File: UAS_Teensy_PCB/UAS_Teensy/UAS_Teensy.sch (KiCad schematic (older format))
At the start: 9 parts, among them J1 UAS-rescue_SM02B-PASS-TBT(LF)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, J2 SM04B-GHS-TB(LF)(SN)-, J3 SM07B-GHS-TB(LF)(SN), J4 SM07B-GHS-TB(LF)(SN), J5 SM04B-GHS-TB(LF)(SN)-, J6 SM04B-GHS-TB(LF)(SN)-, J7 SM04B-GHS-TB(LF)(SN)-, U1 Teensy4.0, U2 BNO055

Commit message: Teensy Board Updates
Teensy Board Updates
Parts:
- J3, J4: footprint JST_SM07B-GHS-TB(LF)(SN) -> UAS_Teensy:JST_SM08B-GHS-TB(LF)(SN)
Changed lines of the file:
@@
 EESchema Schematic File Version 4
+LIBS:UAS_Teensy-cache
 EELAYER 30 0
 EELAYER END
@@
 F 0 "J3" H 3733 2415 50  0000 C CNN
 F 1 "SM07B-GHS-TB(LF)(SN)" H 3733 2324 50  0000 C CNN
-F 2 "JST_SM07B-GHS-TB(LF)(SN)" H 3500 1800 50  0001 L BNN
+F 2 "UAS_Teensy:JST_SM08B-GHS-TB(LF)(SN)" H 3500 1800 50  0001 L BNN
 F 3 "" H 3500 1800 50  0001 L BNN
 F 4 "MANUFACTURER STANDARD" H 3500 1800 50  0001 L BNN "STANDARD"
@@
 F 0 "J4" H 3233 3015 50  0000 C CNN
 F 1 "SM07B-GHS-TB(LF)(SN)" H 3233 2924 50  0000 C CNN
-F 2 "JST_SM07B-GHS-TB(LF)(SN)" H 3000 2400 50  0001 L BNN
+F 2 "UAS_Teensy:JST_SM08B-GHS-TB(LF)(SN)" H 3000 2400 50  0001 L BNN
 F 3 "" H 3000 2400 50  0001 L BNN
 F 4 "MANUFACTURER STANDARD" H 3000 2400 50  0001 L BNN "STANDARD"

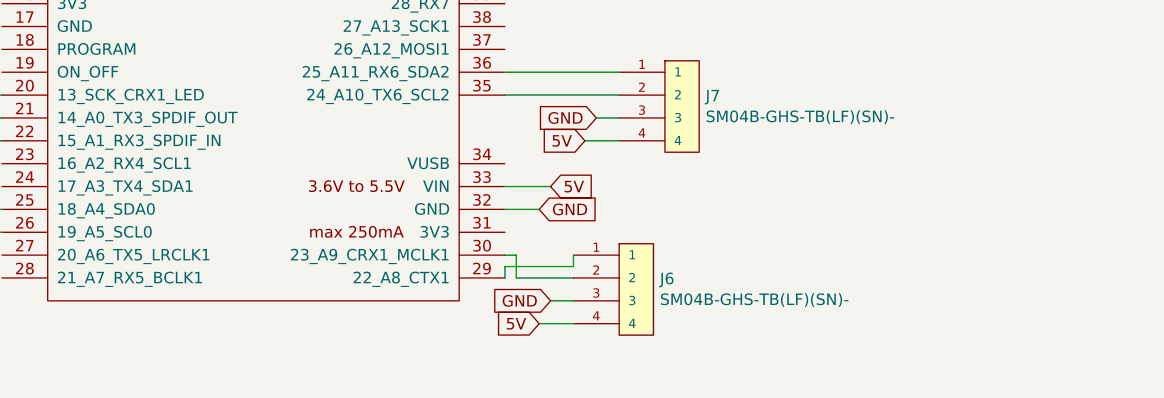
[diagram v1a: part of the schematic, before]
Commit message: For Realsies Final Teensy PCB
lol
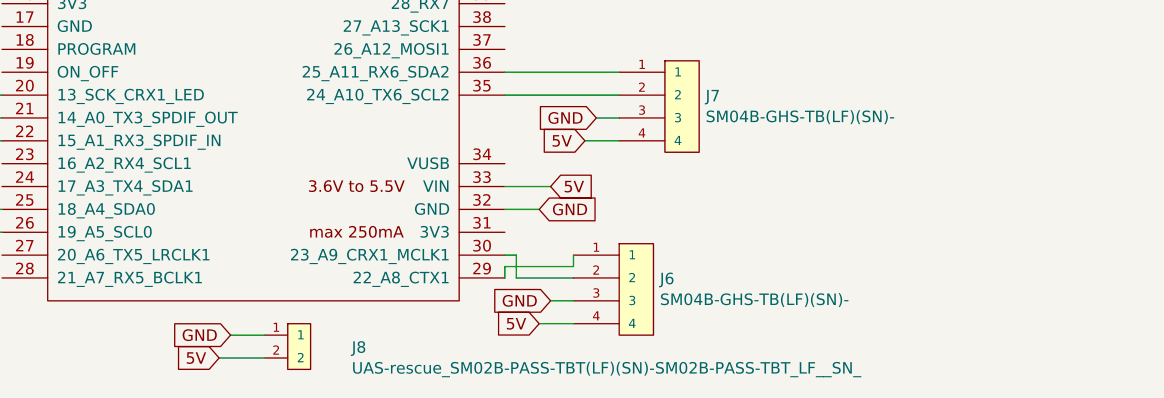
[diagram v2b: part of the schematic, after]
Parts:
- added J8: UAS-rescue_SM02B-PASS-TBT(LF)(SN)-SM02B-PASS-TBT_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, UAS_Teensy:SM02BGHSTBLFSN, symbol UAS:UAS-rescue_SM02B-PASS-TBT(LF)(SN)-SM02B-PASS-TBT_LF__SN_
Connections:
- net +5V: now also J8.2
- net GND: now also J8.1
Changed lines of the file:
@@
 	1    0    0    -1
 $EndComp
-Text GLabel 6550 3700 2    50   Input ~ 0
-5V
-Text GLabel 6500 3800 2    50   Input ~ 0
+Text GLabel 5150 4350 0    50   Input ~ 0
 GND
-Wire Wire Line
-	6550 3700 6350 3700
-Wire Wire Line
-	6500 3800 6350 3800
 Wire Wire Line
 	6750 2700 6750 2800
@@
 	6850 3400 6750 3400
 Wire Wire Line
-	6700 3500 6850 3500
-Wire Wire Line
 	6350 3200 6850 3200
 Wire Wire Line
@@
 Text GLabel 3800 4000 2    50   Input ~ 0
 GND
+$Comp
+L UAS:UAS-rescue_SM02B-PASS-TBT(LF)(SN)-SM02B-PASS-TBT_LF__SN_ J8
+U 1 1 607973F1
+P 5450 4400
+F 0 "J8" H 5680 4396 50  0000 L CNN
+F 1 "UAS-rescue_SM02B-PASS-TBT(LF)(SN)-SM02B-PASS-TBT_LF__SN_" H 5680 4305 50  0000 L CNN
+F 2 "UAS_Teensy:SM02BGHSTBLFSN" H 5450 4400 50  0001 L BNN
+F 3 "" H 5450 4400 50  0001 L BNN
+F 4 "N/A" H 5450 4400 50  0001 L BNN "PARTREV"
+F 5 "JST" H 5450 4400 50  0001 L BNN "MANUFACTURER"
+F 6 "Manufacturer Recommendations" H 5450 4400 50  0001 L BNN "STANDARD"
+F 7 "5.7 mm" H 5450 4400 50  0001 L BNN "MAXIMUM_PACKAGE_HEIGHT"
+	1    5450 4400
+	1    0    0    -1
+$EndComp
+Wire Wire Line
+	6700 3500 6850 3500
+Text GLabel 5100 4450 0    50   Input ~ 0
+5V
+Wire Wire Line
+	5300 4350 5150 4350
+Wire Wire Line
+	5300 4450 5100 4450
+Text GLabel 6500 3800 2    50   Input ~ 0
+GND
+Text GLabel 6550 3700 2    50   Input ~ 0
+5V
+Wire Wire Line
+	6350 3800 6500 3800
+Wire Wire Line
+	6350 3700 6550 3700
 $EndSCHEMATC

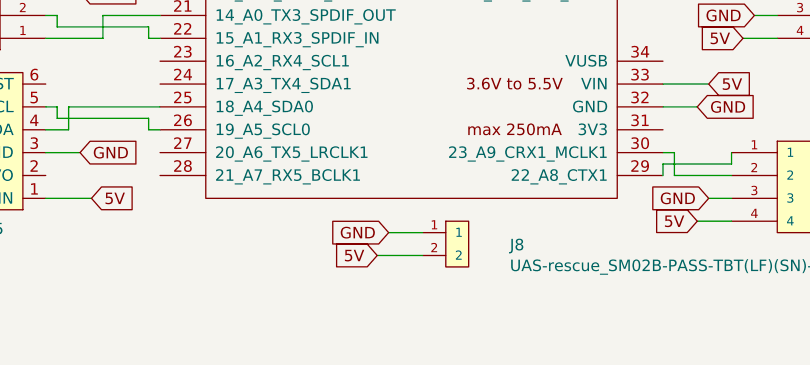
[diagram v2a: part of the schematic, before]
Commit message: final version
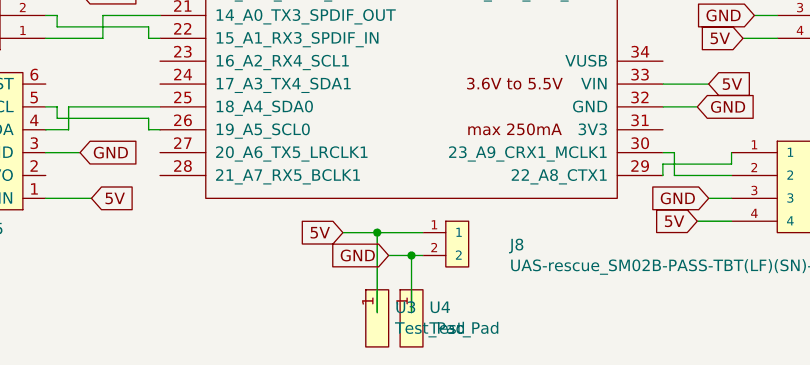
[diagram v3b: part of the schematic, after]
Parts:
- added U3, U4: Test_Pad, UAS_Teensy:Individual_Solder_Pad, symbol UAS_Teensy:Test_Pad
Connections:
- net +5V: now also J8.1, U3.1; no longer J8.2
- net GND: now also J8.2, U4.1; no longer J8.1
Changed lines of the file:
@@
 EESchema Schematic File Version 4
-LIBS:UAS_Teensy-cache
 EELAYER 30 0
 EELAYER END
@@
 	1    0    0    -1
 $EndComp
-Text GLabel 5150 4350 0    50   Input ~ 0
+Text GLabel 5150 4450 0    50   Input ~ 0
 GND
 Wire Wire Line
@@
 Wire Wire Line
 	6700 3500 6850 3500
-Text GLabel 5100 4450 0    50   Input ~ 0
-5V
-Wire Wire Line
-	5300 4350 5150 4350
-Wire Wire Line
-	5300 4450 5100 4450
+Text GLabel 4950 4350 0    50   Input ~ 0
+5V
+Wire Wire Line
+	5300 4450 5250 4450
 Text GLabel 6500 3800 2    50   Input ~ 0
 GND
@@
 Wire Wire Line
 	6350 3700 6550 3700
+$Comp
+L UAS_Teensy:Test_Pad U4
+U 1 1 607AED00
+P 5250 4500
+F 0 "U4" H 5328 4322 50  0000 L CNN
+F 1 "Test_Pad" H 5328 4231 50  0000 L CNN
+F 2 "UAS_Teensy:Individual_Solder_Pad" H 5250 4500 50  0001 C CNN
+F 3 "" H 5250 4500 50  0001 C CNN
+	1    5250 4500
+	1    0    0    -1
+$EndComp
+Wire Wire Line
+	5250 4450 5250 4700
+Connection ~ 5250 4450
+Wire Wire Line
+	5250 4450 5150 4450
+$Comp
+L UAS_Teensy:Test_Pad U3
+U 1 1 607B1DE3
+P 5100 4500
+F 0 "U3" H 5178 4322 50  0000 L CNN
+F 1 "Test_Pad" H 5178 4231 50  0000 L CNN
+F 2 "UAS_Teensy:Individual_Solder_Pad" H 5100 4500 50  0001 C CNN
+F 3 "" H 5100 4500 50  0001 C CNN
+	1    5100 4500
+	1    0    0    -1
+$EndComp
+Wire Wire Line
+	4950 4350 5100 4350
+Wire Wire Line
+	5100 4350 5100 4700
+Connection ~ 5100 4350
+Wire Wire Line
+	5100 4350 5300 4350
 $EndSCHEMATC
